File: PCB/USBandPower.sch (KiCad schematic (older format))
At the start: 16 parts

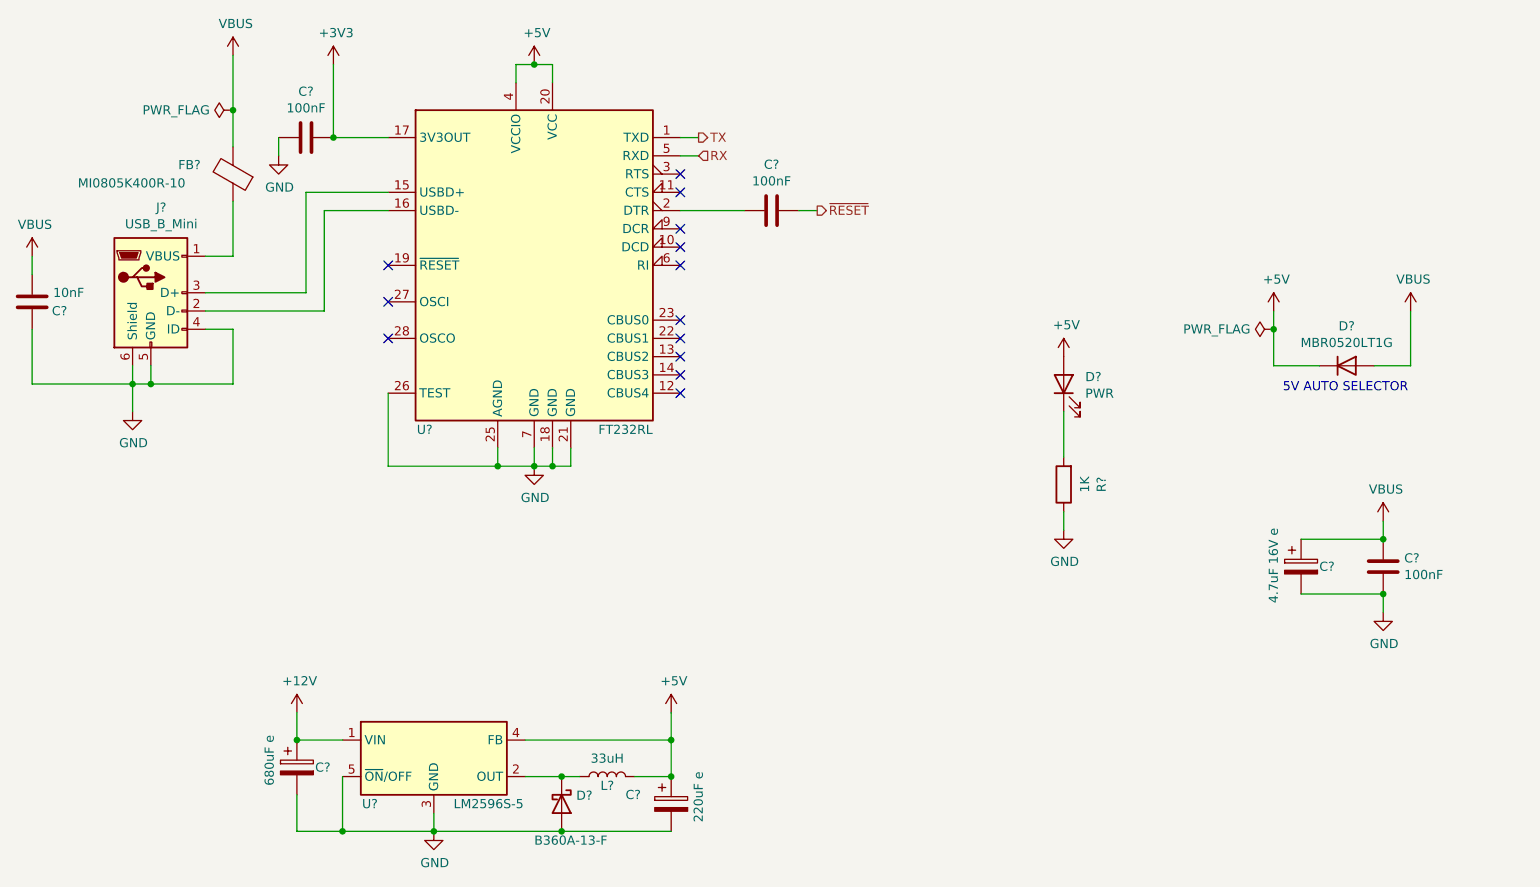
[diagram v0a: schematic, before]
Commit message: WIP
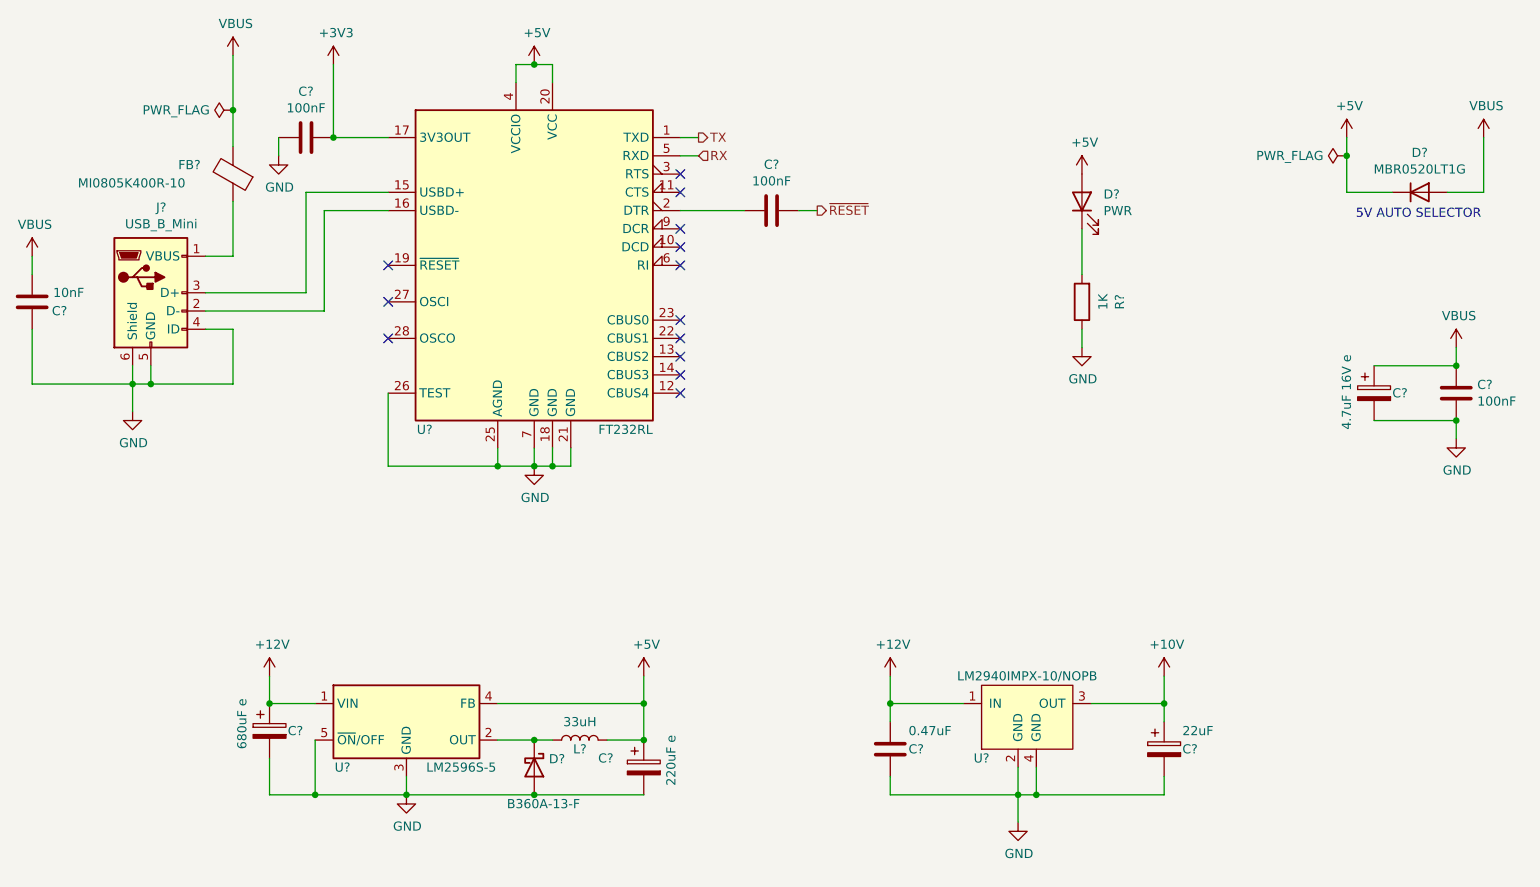
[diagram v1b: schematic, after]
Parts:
- added C?: 22uF, Capacitor_SMD:CP_Elec_10x10.5, symbol Device:CP
- added C?: 0.47uF, Capacitor_SMD:C_0805_2012Metric, symbol Device:C
- added U?: LM2940, Package_TO_SOT_SMD:SOT-223, symbol BritishIdeas:LM2940
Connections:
- net +12V: now also C?.1, U?.1 (IN)
- net GND: now also C?.2, C?.2, U?.2 (GND), U?.4 (GND)
- new net +10V: C?.1, U?.3 (OUT)
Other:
- moved on the sheet: C?, D?, L?, R?, U?
